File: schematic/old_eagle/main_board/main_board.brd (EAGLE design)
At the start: 16 parts, among them IC1 LM1117MPX-5.0, J1 POWER_JACK, U1 STM32L151C6T6

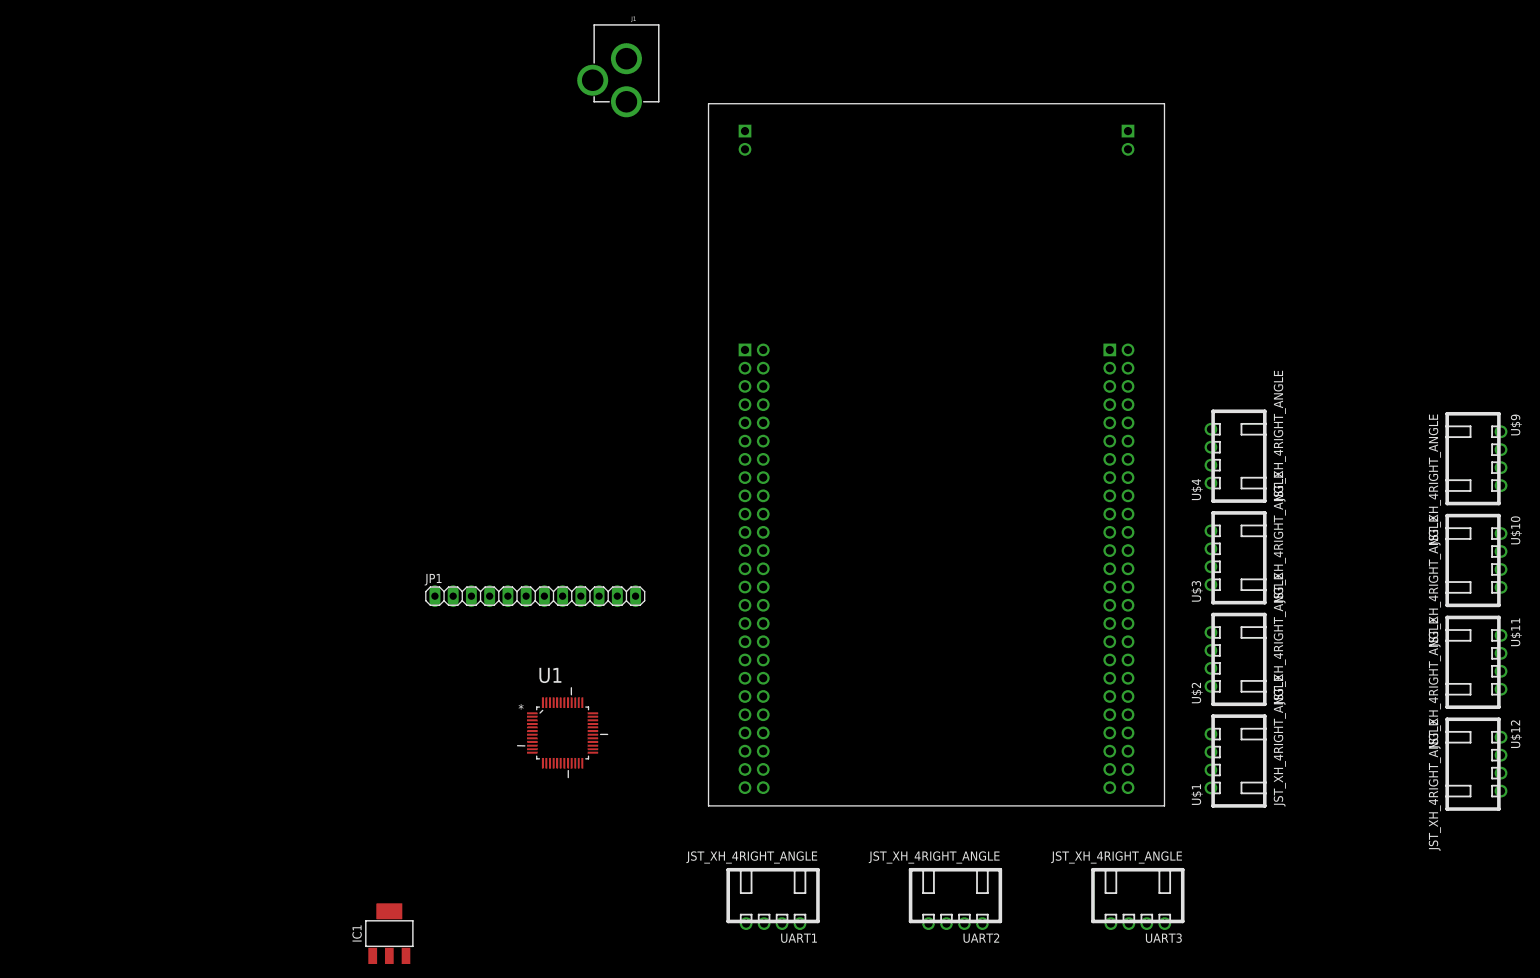
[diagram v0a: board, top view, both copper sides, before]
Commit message: Committing everything
Because my hard drive will soon crash and burn.o
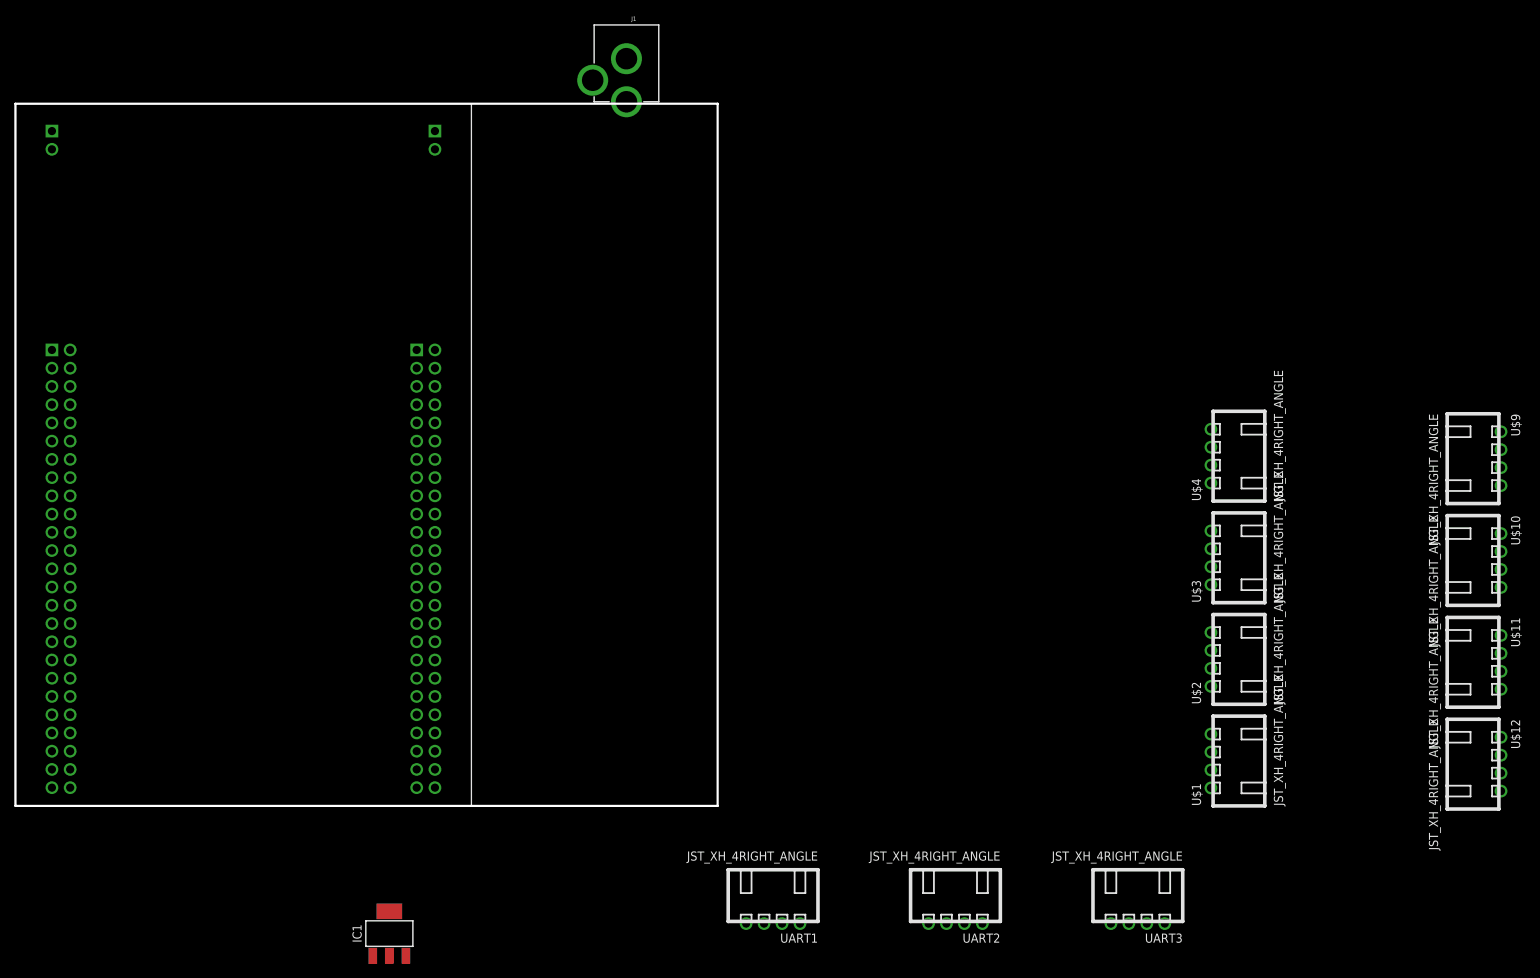
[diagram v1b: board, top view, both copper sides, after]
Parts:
- removed JP1: (no value), pinhead:1X12
- removed U1: STM32L151C6T6, ST Microelctronics_By_element14_Batch_1:QFP50P900X900X160-48N
- moved STM32F411DISC 96.5 mm to (31.8, 35.6)
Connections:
- removed net VDDA: U1.9
- removed net VDD_1: U1.24
- removed net VDD_2: U1.36
- removed net VDD_3: U1.48
- removed net VLCD: U1.1
- removed net VSSA: U1.8
- removed net VSS_1: U1.23
- removed net VSS_2: U1.35
- removed net VSS_3: U1.47
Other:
- board outline added: 97.8 x 97.8 mm
